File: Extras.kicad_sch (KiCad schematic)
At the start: 2 parts, among them J2 RGBLED

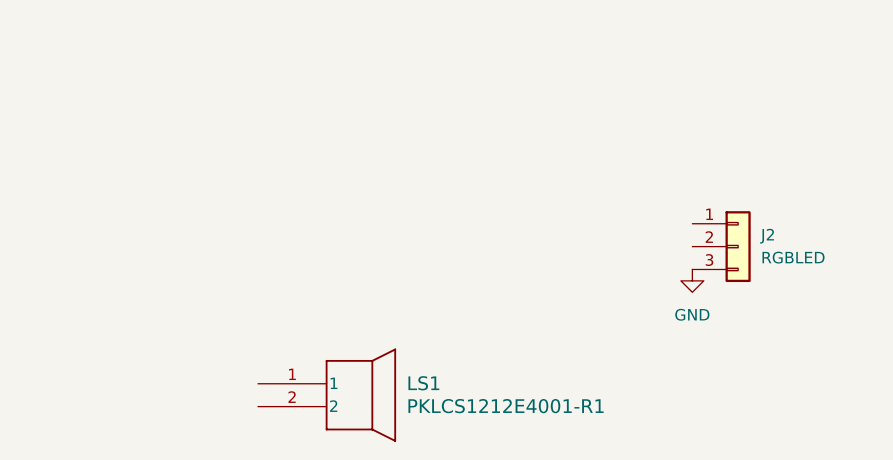
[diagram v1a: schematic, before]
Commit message: Lots of changes
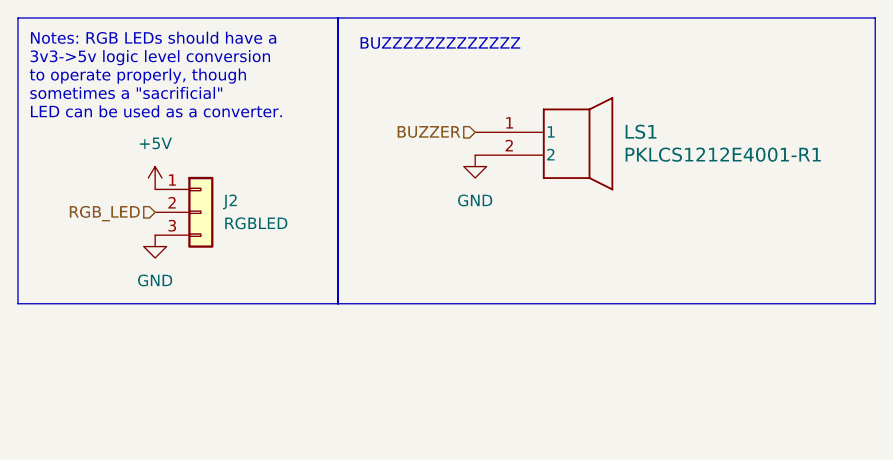
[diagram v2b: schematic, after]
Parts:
- J2: footprint (none) -> Connector_PinHeader_2.54mm:PinHeader_1x03_P2.54mm_Vertical
- LS1: footprint PKLCS_472x472_MUR -> Buzzer_Beeper:Buzzer_12x9.5RM7.6
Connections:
- net GND: now also LS1.2
- net BUZZER: now reaches LS1.1
- net +5V: now reaches J2.1 (Pin_1)
- net RGB_LED: now reaches J2.2 (Pin_2)
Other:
- note added: "BUZZZZZZZZZZZZZ"
- note added: "Notes: RGB LEDs should have a 3v3->5v logic level conversion to operate properly, though sometimes a "sacrificial" LED can be used as a converter."
- moved on the sheet: J2, LS1
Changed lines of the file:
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@@
 (kicad_sch (version 20230121) (generator eeschema)
   (paper "A4")
-  (symbol (lib_id "PKLCS1212E4001:PKLCS1212E4001-R1") (at 39.37 53.34 0) (unit 1)
+  (rectangle (start 12.7 12.7) (end 48.26 44.45)
+    (stroke (width 0) (type default))
+    (fill (type none))
+  )
+  (rectangle (start 48.26 12.7) (end 107.95 44.45)
+    (stroke (width 0) (type default))
+    (fill (type none))
+  )
+  (text "BUZZZZZZZZZZZZZ" (at 68.58 16.51 0)
+    (effects (font (size 1.27 1.27)) (justify right bottom))
+  )
+  (text "Notes: RGB LEDs should have a\n3v3->5v logic level conversion\nto operate properly, though\nsometimes a \"sacrificial\"\nLED can be used as a converter."
+    (at 13.97 24.13 0)
+    (effects (font (size 1.27 1.27)) (justify left bottom))
+  )
+  (hierarchical_label "BUZZER" (shape input) (at 63.5 25.4 180) (fields_autoplaced)
+    (effects (font (size 1.27 1.27)) (justify right))
+  )
+  (hierarchical_label "RGB_LED" (shape input) (at 27.94 34.29 180) (fields_autoplaced)
+    (effects (font (size 1.27 1.27)) (justify right))
+  )
+  (symbol (lib_id "PKLCS1212E4001:PKLCS1212E4001-R1") (at 63.5 25.4 0) (unit 1)
     (in_bom yes) (on_board yes) (dnp no) (fields_autoplaced)
-    (property "Reference" "LS1" (at 55.88 53.34 0)
+    (property "Reference" "LS1" (at 80.01 25.4 0)
       (effects (font (size 1.524 1.524)) (justify left))
     )
-    (property "Value" "PKLCS1212E4001-R1" (at 55.88 55.88 0)
+    (property "Value" "PKLCS1212E4001-R1" (at 80.01 27.94 0)
       (effects (font (size 1.524 1.524)) (justify left))
     )
-    (property "Footprint" "PKLCS_472x472_MUR" (at 39.37 53.34 0)
+    (property "Footprint" "Buzzer_Beeper:Buzzer_12x9.5RM7.6" (at 63.5 25.4 0)
       (effects (font (size 1.27 1.27) italic) hide)
     )
-    (property "Datasheet" "PKLCS1212E4001-R1" (at 39.37 53.34 0)
+    (property "Datasheet" "PKLCS1212E4001-R1" (at 63.5 25.4 0)
       (effects (font (size 1.27 1.27) italic) hide)
     )
@@
     )
   )
-  (symbol (lib_id "power:GND") (at 87.63 40.64 0) (unit 1)
+  (symbol (lib_id "power:GND") (at 63.5 27.94 0) (unit 1)
     (in_bom yes) (on_board yes) (dnp no) (fields_autoplaced)
-    (property "Reference" "#PWR05" (at 87.63 46.99 0)
+    (property "Reference" "#PWR048" (at 63.5 34.29 0)
       (effects (font (size 1.27 1.27)) hide)
     )
-    (property "Value" "GND" (at 87.63 45.72 0)
+    (property "Value" "GND" (at 63.5 33.02 0)
       (effects (font (size 1.27 1.27)))
     )
-    (property "Footprint" "" (at 87.63 40.64 0)
+    (property "Footprint" "" (at 63.5 27.94 0)
       (effects (font (size 1.27 1.27)) hide)
     )
-    (property "Datasheet" "" (at 87.63 40.64 0)
+    (property "Datasheet" "" (at 63.5 27.94 0)
+      (effects (font (size 1.27 1.27)) hide)
+    )
+    (pin "1")
+    (instances
+      (project "Pico-Skidi"
+        (path "/21865b85-eb74-4d61-a31a-30858d3bc341/a918f8c6-b50a-4fb5-8fe4-4f099461944c"
+          (reference "#PWR048") (unit 1)
+        )
+      )
+    )
+  )
+  (symbol (lib_id "power:+5V") (at 27.94 31.75 0) (unit 1)
+    (in_bom yes) (on_board yes) (dnp no) (fields_autoplaced)
+    (property "Reference" "#PWR046" (at 27.94 35.56 0)
+      (effects (font (size 1.27 1.27)) hide)
+    )
+    (property "Value" "+5V" (at 27.94 26.67 0)
+      (effects (font (size 1.27 1.27)))
+    )
+    (property "Footprint" "" (at 27.94 31.75 0)
+      (effects (font (size 1.27 1.27)) hide)
+    )
+    (property "Datasheet" "" (at 27.94 31.75 0)
+      (effects (font (size 1.27 1.27)) hide)
+    )
+    (pin "1")
+    (instances
+      (project "Pico-Skidi"
+        (path "/21865b85-eb74-4d61-a31a-30858d3bc341/a918f8c6-b50a-4fb5-8fe4-4f099461944c"
+          (reference "#PWR046") (unit 1)
+        )
+      )
+    )
+  )
+  (symbol (lib_id "power:GND") (at 27.94 36.83 0) (unit 1)
+    (in_bom yes) (on_board yes) (dnp no) (fields_autoplaced)
+    (property "Reference" "#PWR05" (at 27.94 43.18 0)
+      (effects (font (size 1.27 1.27)) hide)
+    )
+    (property "Value" "GND" (at 27.94 41.91 0)
+      (effects (font (size 1.27 1.27)))
+    )
+    (property "Footprint" "" (at 27.94 36.83 0)
+      (effects (font (size 1.27 1.27)) hide)
+    )
+    (property "Datasheet" "" (at 27.94 36.83 0)
       (effects (font (size 1.27 1.27)) hide)
     )
@@
         )
         (path "/21865b85-eb74-4d61-a31a-30858d3bc341/a918f8c6-b50a-4fb5-8fe4-4f099461944c"
-          (reference "#PWR05") (unit 1)
+          (reference "#PWR047") (unit 1)
         )
       )
     )
   )
-  (symbol (lib_id "Connector_Generic:Conn_01x03") (at 92.71 38.1 0) (unit 1)
+  (symbol (lib_id "Connector_Generic:Conn_01x03") (at 33.02 34.29 0) (unit 1)
     (in_bom yes) (on_board yes) (dnp no) (fields_autoplaced)
-    (property "Reference" "J2" (at 95.25 36.83 0)
+    (property "Reference" "J2" (at 35.56 33.02 0)
       (effects (font (size 1.27 1.27)) (justify left))
     )
-    (property "Value" "RGBLED" (at 95.25 39.37 0)
+    (property "Value" "RGBLED" (at 35.56 35.56 0)
       (effects (font (size 1.27 1.27)) (justify left))
     )
-    (property "Footprint" "" (at 92.71 38.1 0)
+    (property "Footprint" "Connector_PinHeader_2.54mm:PinHeader_1x03_P2.54mm_Vertical" (at 33.02 34.29 0)
       (effects (font (size 1.27 1.27)) hide)
     )
-    (property "Datasheet" "~" (at 92.71 38.1 0)
+    (property "Datasheet" "~" (at 33.02 34.29 0)
       (effects (font (size 1.27 1.27)) hide)
     )
@@
         )
         (path "/21865b85-eb74-4d61-a31a-30858d3bc341/a918f8c6-b50a-4fb5-8fe4-4f099461944c"
-          (reference "J2") (unit 1)
+          (reference "J16") (unit 1)
         )
       )

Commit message: syncing
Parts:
- LS1: footprint Buzzer_Beeper:Buzzer_12x9.5RM7.6 -> PKLCS1212:PKLCS_472x472_MUR
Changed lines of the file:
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@@
       (effects (font (size 1.524 1.524)) (justify left))
     )
-    (property "Footprint" "Buzzer_Beeper:Buzzer_12x9.5RM7.6" (at 63.5 25.4 0)
+    (property "Footprint" "PKLCS1212:PKLCS_472x472_MUR" (at 63.5 25.4 0)
       (effects (font (size 1.27 1.27) italic) hide)
     )
@@
   (symbol (lib_id "power:GND") (at 63.5 27.94 0) (unit 1)
     (in_bom yes) (on_board yes) (dnp no) (fields_autoplaced)
-    (property "Reference" "#PWR048" (at 63.5 34.29 0)
+    (property "Reference" "#PWR051" (at 63.5 34.29 0)
       (effects (font (size 1.27 1.27)) hide)
     )
@@
       (project "Pico-Skidi"
         (path "/21865b85-eb74-4d61-a31a-30858d3bc341/a918f8c6-b50a-4fb5-8fe4-4f099461944c"
-          (reference "#PWR048") (unit 1)
+          (reference "#PWR051") (unit 1)
         )
       )
@@
   (symbol (lib_id "power:+5V") (at 27.94 31.75 0) (unit 1)
     (in_bom yes) (on_board yes) (dnp no) (fields_autoplaced)
-    (property "Reference" "#PWR046" (at 27.94 35.56 0)
+    (property "Reference" "#PWR049" (at 27.94 35.56 0)
       (effects (font (size 1.27 1.27)) hide)
     )
@@
       (project "Pico-Skidi"
         (path "/21865b85-eb74-4d61-a31a-30858d3bc341/a918f8c6-b50a-4fb5-8fe4-4f099461944c"
-          (reference "#PWR046") (unit 1)
+          (reference "#PWR049") (unit 1)
         )
       )
@@
         )
         (path "/21865b85-eb74-4d61-a31a-30858d3bc341/a918f8c6-b50a-4fb5-8fe4-4f099461944c"
-          (reference "#PWR047") (unit 1)
+          (reference "#PWR050") (unit 1)
         )
       )
@@
         )
         (path "/21865b85-eb74-4d61-a31a-30858d3bc341/a918f8c6-b50a-4fb5-8fe4-4f099461944c"
-          (reference "J16") (unit 1)
+          (reference "J9") (unit 1)
         )
       )
